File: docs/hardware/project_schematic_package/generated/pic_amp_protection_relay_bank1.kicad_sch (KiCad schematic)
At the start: 14 parts, among them K1 160m, K2 80m, K3 40m, K4 20m, K5 15m, K6 10m, K7 6m

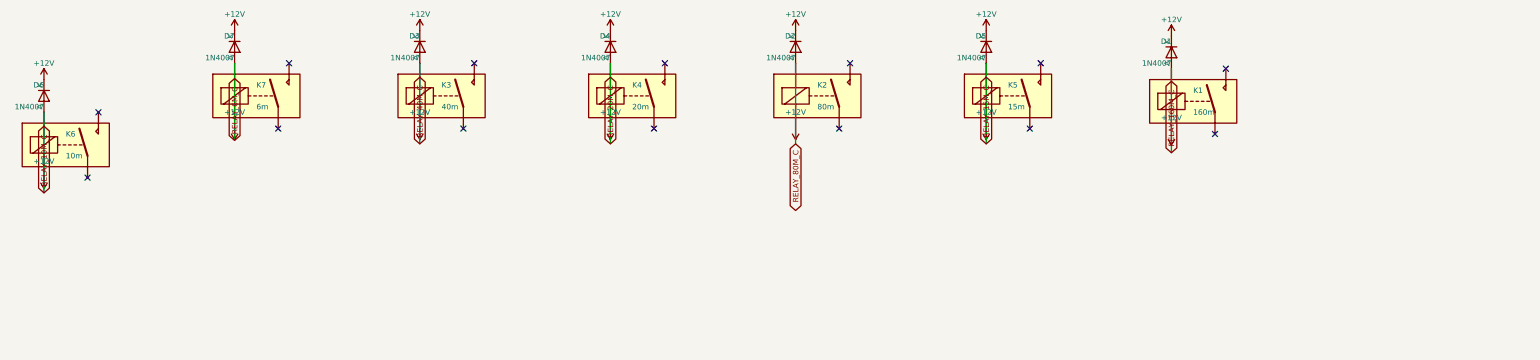
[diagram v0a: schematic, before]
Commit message: Add structured schematic generation rules
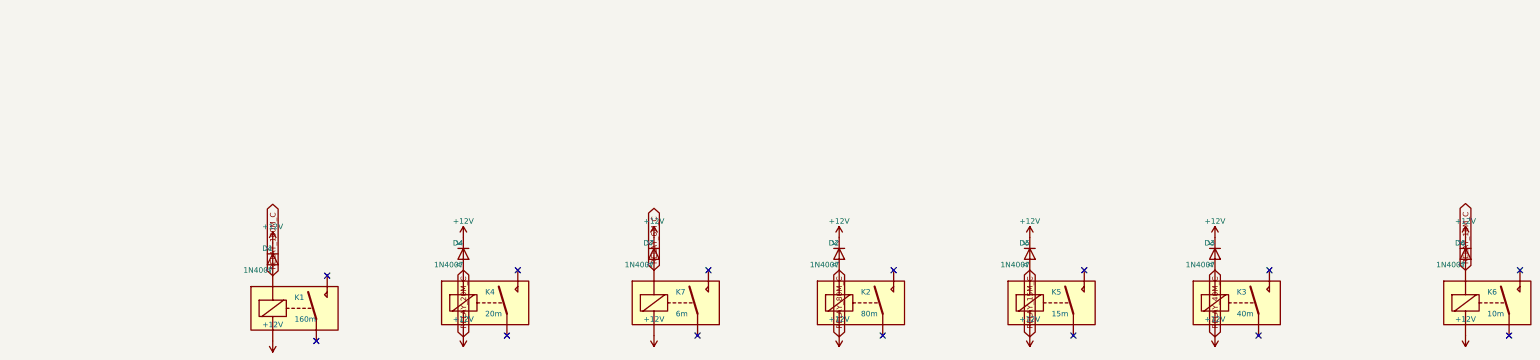
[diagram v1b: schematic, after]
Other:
- moved on the sheet: D1, D2, D3, D4, D5, D6, D7, K1, K2, K3, K4, K5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

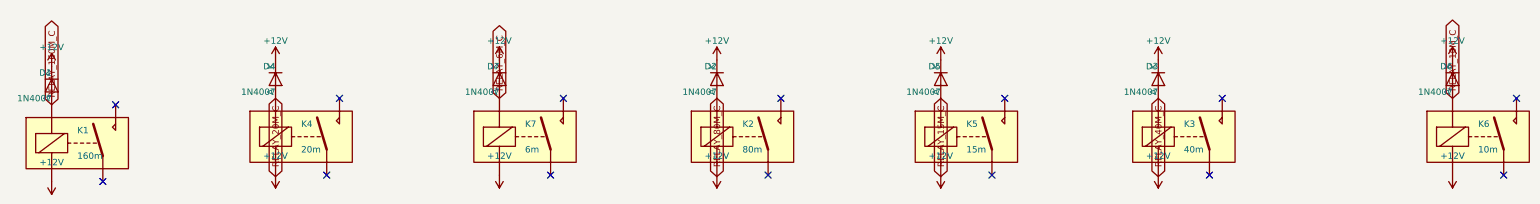
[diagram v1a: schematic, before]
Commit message: Update schematic generation work
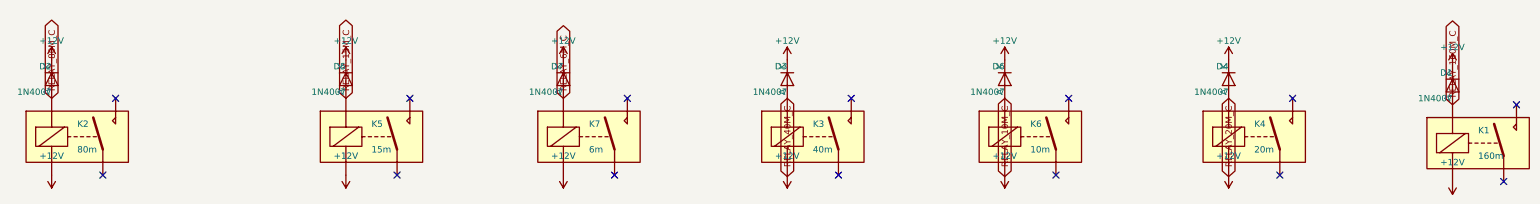
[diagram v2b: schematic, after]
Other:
- moved on the sheet: D1, D2, D3, D4, D5, D6, D7, K1, K2, K3, K4, K5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
